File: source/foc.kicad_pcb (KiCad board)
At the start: 2 copper layers, 68 x 79 mm, 218 parts, among them J1 Conn_01x04_Male, J2 TYPE-C-31-M-12, P1 SWD, Q1 MMBT5401, Q10 CSD19536KCS, Q11 CSD19536KCS, Q12 CSD19536KCS, Q13 MMBT5401, Q14 MMBT5401, Q15 CSD19536KCS, Q16 CSD19536KCS, Q17 CSD19536KCS, Q18 CSD19536KCS, Q2 MMBT5401, Q3 NCEP60T20, Q4 CSD19536KCS, Q5 CSD19536KCS, Q6 CSD19536KCS, Q7 MMBT5401, Q8 MMBT5401, Q9 CSD19536KCS, U1 BMI160, U10 HT7550, U11 STM32F405RGT6, U12 AMS1117-3.3, U2 IRS21867S, U3 IRS21867S, U4 IRS21867S, U5 TX4130L/PW2902, U6 MS8311, U7 MS8311, U8 MS8311, U9 TJA1050T/CM,118, Y1 8MHz Crystal Resonator, X5032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

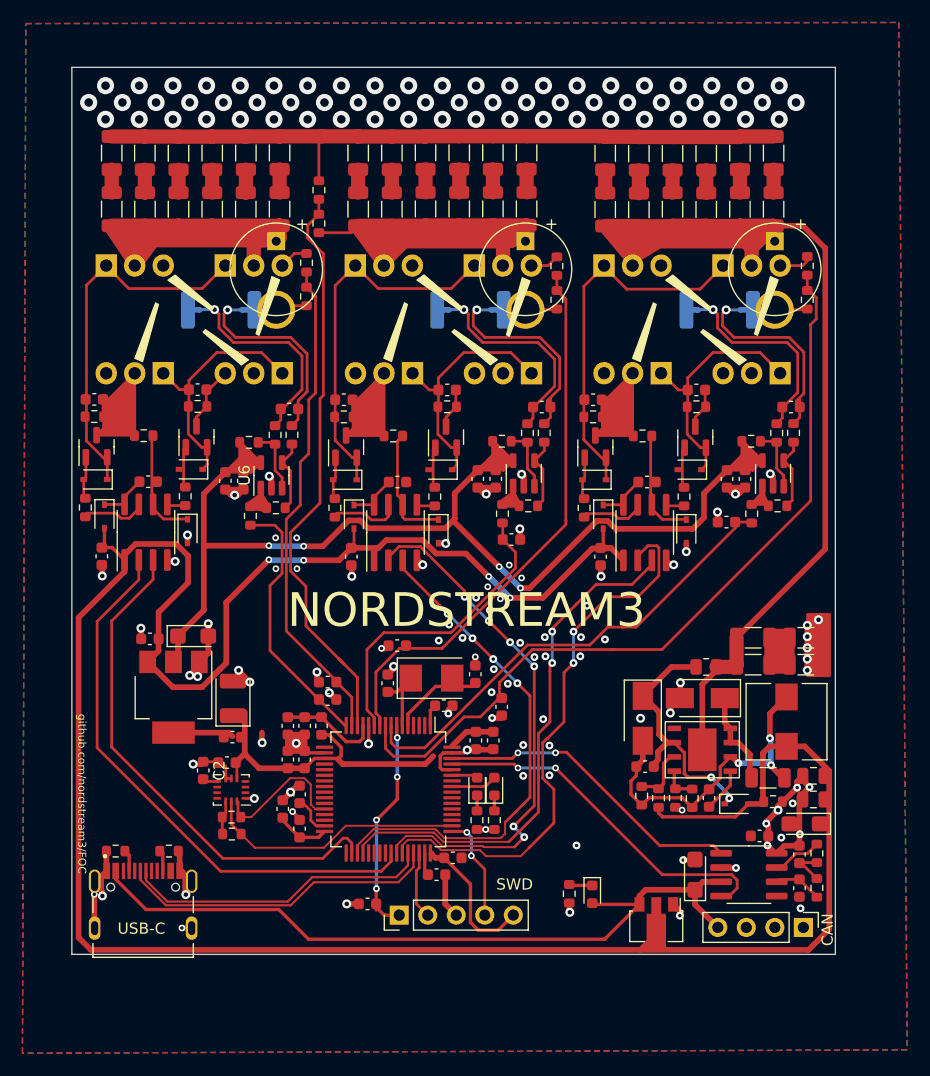
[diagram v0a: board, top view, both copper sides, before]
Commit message: Add files via upload
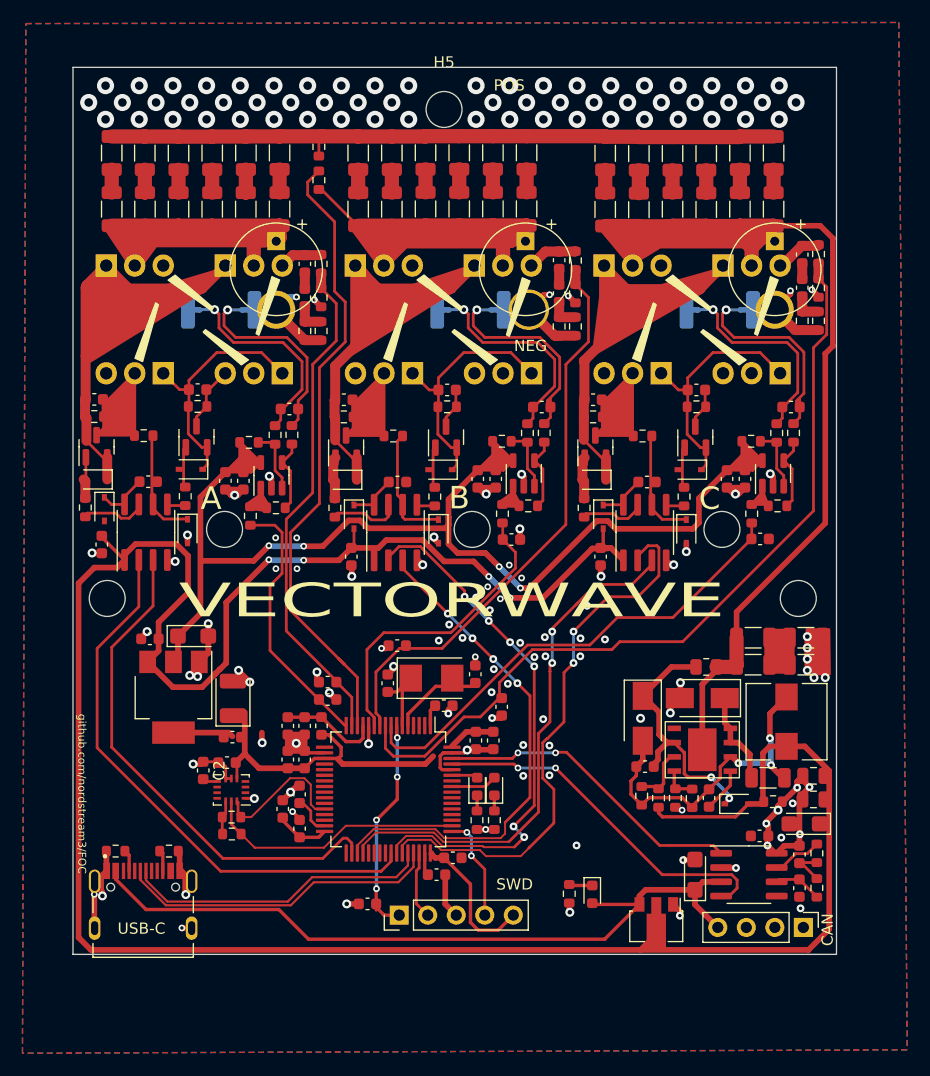
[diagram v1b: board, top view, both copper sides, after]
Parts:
- removed FieldFeets1: R, Custom:field
- added C39: 4.7n, Capacitor_SMD:C_0603_1608Metric, F.Cu at (80.8, 89.5)
- added C41: 4.7n, Capacitor_SMD:C_0603_1608Metric, F.Cu at (80.8, 92.5)
- added C61: 4.7n, Capacitor_SMD:C_0603_1608Metric, F.Cu at (103.4, 89.2)
- added C63: 4.7n, Capacitor_SMD:C_0603_1608Metric, F.Cu at (103.4, 92.1)
- added C82: 4.7n, Capacitor_SMD:C_0603_1608Metric, F.Cu at (125.0, 88.7)
- added C83: 4.7n, Capacitor_SMD:C_0603_1608Metric, F.Cu at (125.0, 91.6)
- added H1: MountingHole, MountingHole:MountingHole_3.2mm_M3, F.Cu at (63.1, 119.3)
- added H2: MountingHole, MountingHole:MountingHole_3.2mm_M3, F.Cu at (117.9, 113.2)
- added H3: MountingHole, MountingHole:MountingHole_3.2mm_M3, F.Cu at (124.7, 119.3)
- added H4: MountingHole, MountingHole:MountingHole_3.2mm_M3, F.Cu at (73.6, 113.2)
- added H5: MountingHole, MountingHole:MountingHole_3.2mm_M3, F.Cu at (93.2, 75.8)
- added H6: MountingHole, MountingHole:MountingHole_3.2mm_M3, F.Cu at (95.7, 113.2)
- added R31: 10R, Resistor_SMD:R_0603_1608Metric, F.Cu at (82.2, 95.5)
- added R32: 10R, Resistor_SMD:R_0603_1608Metric, F.Cu at (80.8, 95.5)
- added R45: 10R, Resistor_SMD:R_0603_1608Metric, F.Cu at (103.4, 95.1)
- added R46: 10R, Resistor_SMD:R_0603_1608Metric, F.Cu at (104.8, 95.1)
- added R57: 10R, Resistor_SMD:R_0603_1608Metric, F.Cu at (126.5, 94.6)
- added R58: 10R, Resistor_SMD:R_0603_1608Metric, F.Cu at (125.0, 94.6)
- moved R6 3.85 mm to (82.0, 82.0)
- moved R7 3.85 mm to (82.0, 79.1)
- moved C65 3.35 mm to (121.3, 114.0), turned to 180 degrees
- moved R9 1.74 mm to (104.8, 92.2)
- moved R8 1.72 mm to (104.8, 89.2)
- moved R12 1.45 mm to (126.5, 88.6)
- moved R13 1.45 mm to (126.5, 91.7)
- moved R3 1.30 mm to (82.2, 89.5)
- moved R4 1.30 mm to (82.2, 92.5)
- moved C3 1.05 mm to (62.7, 114.5)
- moved D1 0.65 mm to (62.9, 111.3)
- renumbered C98 to C100, C99 to C101, C101 to C103, C102 to C104, C103 to C105, C104 to C106, C105 to C107, C106 to C108, C107 to C109, C17 to C13, C18 to C14, C19 to C15, C20 to C16, C21 to C17, C22 to C18, C23 to C19, C24 to C20, C25 to C21, C26 to C22, C27 to C23, C28 to C24, C29 to C25, C30 to C26, C31 to C27, C32 to C28, C33 to C29, C34 to C30, C35 to C31, C36 to C32, C37 to C33, C38 to C34, C39 to C35, C40 to C36, C41 to C37, C42 to C38, C43 to C40, C44 to C42, C45 to C43, C47 to C45, C48 to C46, C49 to C47, C50 to C48, C51 to C49, C52 to C50, C53 to C51, C54 to C52, C55 to C53, C56 to C54, C57 to C55, C58 to C56, C59 to C57, C60 to C58, C61 to C59, C62 to C60, C64 to C62, C63 to C64, C82 to C84, C83 to C85, C84 to C86, C85 to C87, C86 to C88, C87 to C89, C88 to C90, C89 to C91, C90 to C92, C91 to C93, C93 to C94, C92 to C95, C94 to C96, C96 to C98, C97 to C99, R31 to R33, R33 to R35, R34 to R36, R35 to R37, R37 to R39, R38 to R40, R39 to R41, R40 to R42, R41 to R43, R42 to R44, R43 to R47, R44 to R48, R45 to R49, R46 to R50, R47 to R51, R48 to R52, R49 to R53, R50 to R54, R51 to R55, R52 to R56, R53 to R59, R54 to R60, R55 to R61, R56 to R62, R57 to R63, R58 to R64, R59 to R65
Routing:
- net Net-(C66-Pad1): track 32.8 -> 54.4 mm
- net Net-(C23-Pad1): track 32.9 -> 51.5 mm
- net GND: track 204.7 -> 212.6 mm, vias 161 -> 162
- net /driver/SENS_SUPPLY: track 52.3 -> 56.5 mm
- net Net-(C45-Pad1): track 33.1 -> 36.8 mm
- net Net-(C41-Pad2): track 0.00 -> 2.83 mm
- net Net-(C83-Pad2): track 0.00 -> 2.80 mm
- net Net-(C63-Pad2): track 0.00 -> 2.80 mm
- net VCC: track 169.9 -> 172.6 mm
- net V_IN: track 132.0 -> 134.6 mm
- net /driver/HS2: track 19.0 -> 20.9 mm
- net /driver/SENS_3: track 71.3 -> 73.1 mm
- net Net-(D14-Pad2): track 3.73 -> 5.46 mm
- net Net-(D10-Pad2): track 3.73 -> 5.46 mm
- net Net-(D12-Pad2): track 3.73 -> 5.46 mm
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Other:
- board text added: "A"
- board text added: "B"
- board text added: "C"
- board text added: "NEG"
- board text added: "POS"
- board text added: "VECTORWAVE"
- board text removed: "NORDSTREAM3"

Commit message: Add files via upload
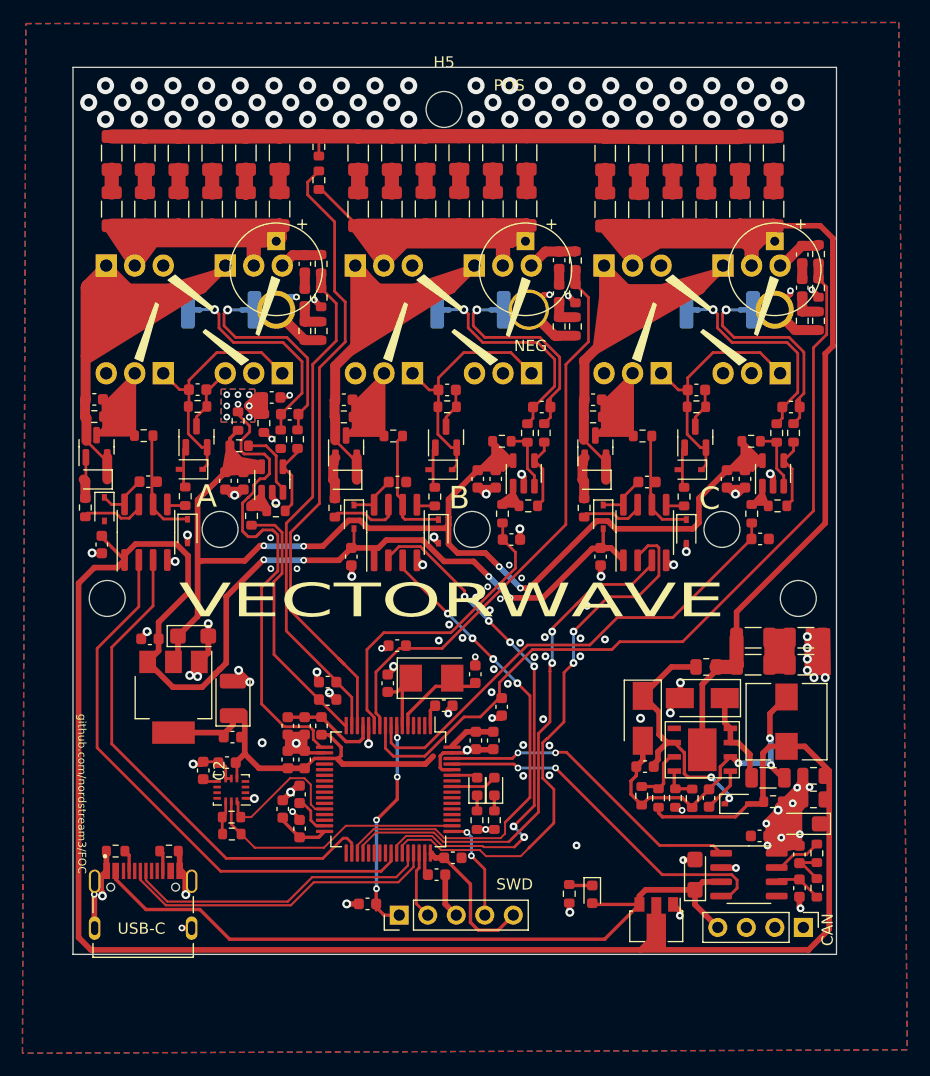
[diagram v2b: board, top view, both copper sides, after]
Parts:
- added C44: 2.2u, Capacitor_SMD:C_0603_1608Metric, F.Cu at (77.8, 101.4)
- added R34: NTC 10k, Resistor_SMD:R_0603_1608Metric, F.Cu at (74.8, 103.5)
- added R38: 10k, Resistor_SMD:R_0603_1608Metric, F.Cu at (77.1, 103.7)
- moved R25 0.92 mm to (74.9, 105.7)
- moved R28 0.63 mm to (78.6, 105.1)
- moved R29 0.63 mm to (80.1, 105.1)
- moved C25 0.47 mm to (79.4, 102.9)
- moved H4 0.40 mm to (73.2, 113.2)
- moved U6 0.38 mm to (77.8, 108.7)
- moved R24 0.28 mm to (78.2, 111.5)
- moved R21 0.10 mm to (76.0, 112.0)
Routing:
- net /mcu/ADC_TEMP: track 0.00 -> 47.7 mm, vias 0 -> 8
- net GND: track 212.6 -> 214.9 mm, vias 162 -> 164
- net Net-(C25-Pad1): track 18.0 -> 18.6 mm
- net VCC: track 172.6 -> 173.3 mm
- net Net-(R25-Pad1): track 5.74 -> 6.34 mm
- net +12V: track 227.6 -> 228.1 mm
- added copper zone on B.Cu, net /mcu/ADC_TEMP
- added copper zone on F.Cu, net /mcu/ADC_TEMP
